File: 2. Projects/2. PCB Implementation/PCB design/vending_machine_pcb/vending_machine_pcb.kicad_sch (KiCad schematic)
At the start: 0 parts

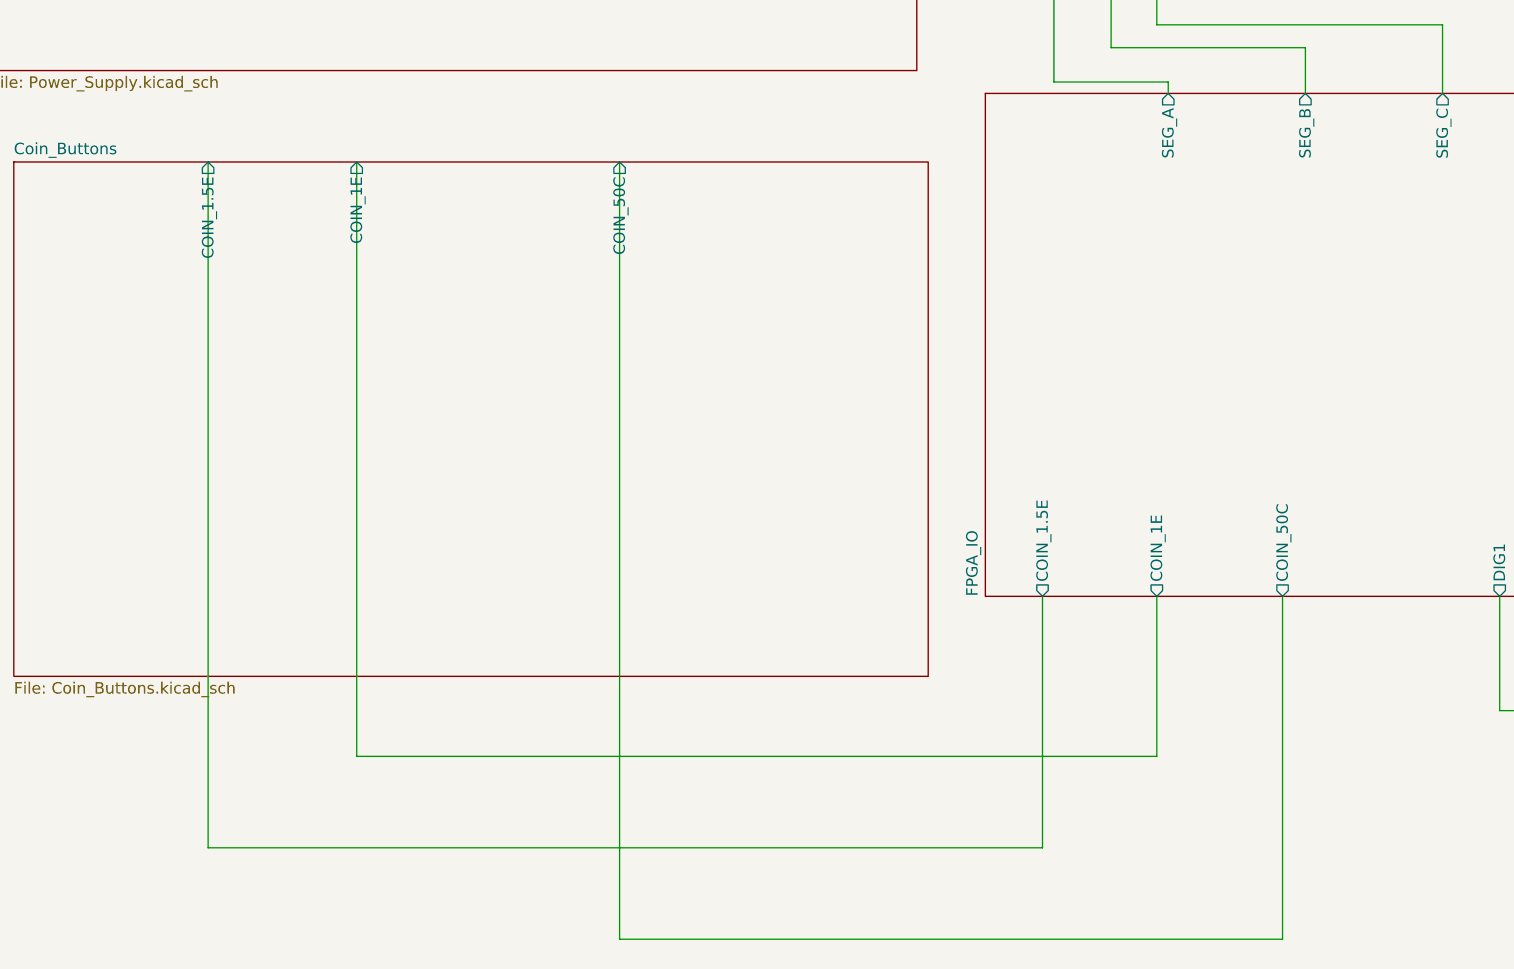
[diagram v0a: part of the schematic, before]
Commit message: PCB implementation
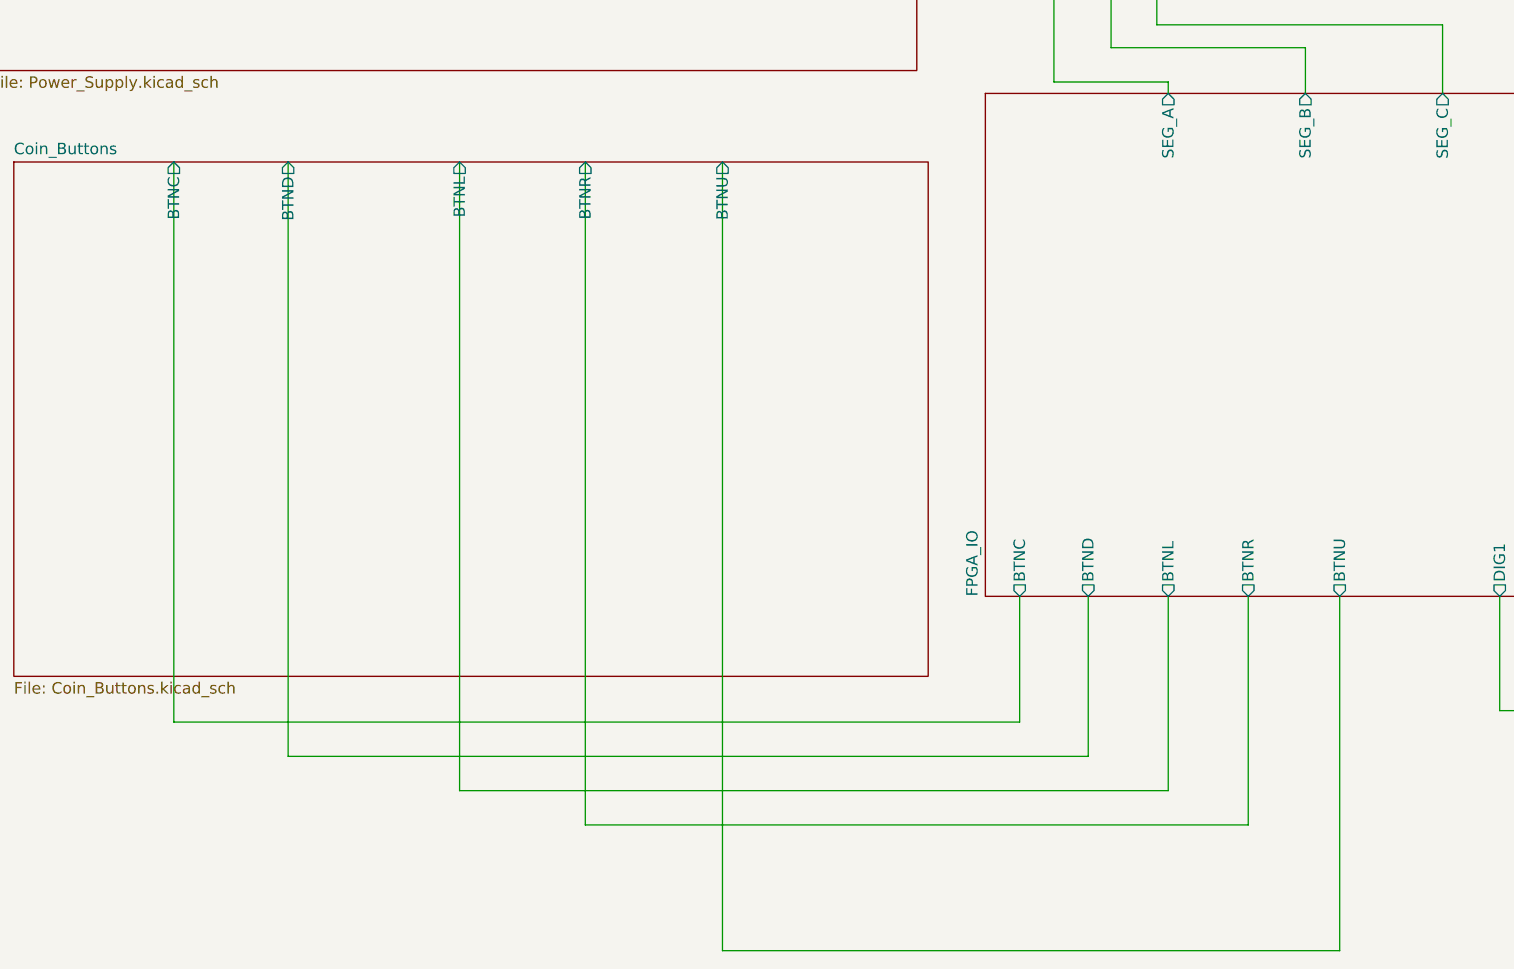
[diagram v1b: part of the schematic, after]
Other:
- sheet Coin_Buttons ports: added BTNC, BTND, BTNL, BTNR, BTNU; removed COIN_1.5E, COIN_1E, COIN_50C
- sheet FPGA_IO ports: added BTNC, BTND, BTNL, BTNR, BTNU; removed COIN_1.5E, COIN_1E, COIN_50C
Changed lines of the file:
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@@
 	(wire
 		(pts
-			(xy 156.21 189.23) (xy 156.21 151.13)
+			(xy 162.56 190.5) (xy 93.98 190.5)
 		)
 		(stroke
@@
 	(wire
 		(pts
+			(xy 78.74 176.53) (xy 152.4 176.53)
+		)
+		(stroke
+			(width 0)
+			(type default)
+		)
+	)
+	(wire
+		(pts
+			(xy 45.72 168.91) (xy 134.62 168.91)
+		)
+		(stroke
+			(width 0)
+			(type default)
+		)
+	)
+	(wire
+		(pts
 			(xy 137.16 90.17) (xy 158.75 90.17)
 		)
@@
 	(wire
 		(pts
-			(xy 53.34 102.87) (xy 53.34 168.91)
+			(xy 33.02 165.1) (xy 127 165.1)
+		)
+		(stroke
+			(width 0)
+			(type default)
+		)
+	)
+	(wire
+		(pts
+			(xy 127 165.1) (xy 127 151.13)
+		)
+		(stroke
+			(width 0)
+			(type default)
+		)
+	)
+	(wire
+		(pts
+			(xy 64.77 102.87) (xy 64.77 172.72)
+		)
+		(stroke
+			(width 0)
+			(type default)
+		)
+	)
+	(wire
+		(pts
+			(xy 162.56 151.13) (xy 162.56 190.5)
 		)
 		(stroke
@@
 	(wire
 		(pts
-			(xy 53.34 168.91) (xy 142.24 168.91)
-		)
-		(stroke
-			(width 0)
-			(type default)
-		)
-	)
-	(wire
-		(pts
 			(xy 130.81 21.59) (xy 130.81 93.98)
 		)
@@
 	(wire
 		(pts
+			(xy 64.77 172.72) (xy 143.51 172.72)
+		)
+		(stroke
+			(width 0)
+			(type default)
+		)
+	)
+	(wire
+		(pts
+			(xy 45.72 102.87) (xy 45.72 168.91)
+		)
+		(stroke
+			(width 0)
+			(type default)
+		)
+	)
+	(wire
+		(pts
 			(xy 226.06 157.48) (xy 226.06 151.13)
 		)
@@
 	(wire
 		(pts
+			(xy 93.98 190.5) (xy 93.98 102.87)
+		)
+		(stroke
+			(width 0)
+			(type default)
+		)
+	)
+	(wire
+		(pts
 			(xy 171.45 21.59) (xy 171.45 52.07)
 		)
@@
 	(wire
 		(pts
-			(xy 142.24 168.91) (xy 142.24 151.13)
-		)
-		(stroke
-			(width 0)
-			(type default)
-		)
-	)
-	(wire
-		(pts
 			(xy 143.51 93.98) (xy 143.51 95.25)
 		)
@@
 	(wire
 		(pts
-			(xy 129.54 179.07) (xy 36.83 179.07)
-		)
-		(stroke
-			(width 0)
-			(type default)
-		)
-	)
-	(wire
-		(pts
 			(xy 283.21 163.83) (xy 180.34 163.83)
 		)
@@
 	(wire
 		(pts
-			(xy 82.55 189.23) (xy 156.21 189.23)
-		)
-		(stroke
-			(width 0)
-			(type default)
-		)
-	)
-	(wire
-		(pts
-			(xy 36.83 179.07) (xy 36.83 102.87)
-		)
-		(stroke
-			(width 0)
-			(type default)
-		)
-	)
-	(wire
-		(pts
-			(xy 129.54 151.13) (xy 129.54 179.07)
+			(xy 33.02 102.87) (xy 33.02 165.1)
 		)
 		(stroke
@@
 	(wire
 		(pts
+			(xy 152.4 176.53) (xy 152.4 151.13)
+		)
+		(stroke
+			(width 0)
+			(type default)
+		)
+	)
+	(wire
+		(pts
 			(xy 276.86 157.48) (xy 226.06 157.48)
 		)
@@
 	(wire
 		(pts
+			(xy 78.74 102.87) (xy 78.74 176.53)
+		)
+		(stroke
+			(width 0)
+			(type default)
+		)
+	)
+	(wire
+		(pts
+			(xy 134.62 168.91) (xy 134.62 151.13)
+		)
+		(stroke
+			(width 0)
+			(type default)
+		)
+	)
+	(wire
+		(pts
 			(xy 200.66 161.29) (xy 280.67 161.29)
 		)
@@
 	(wire
 		(pts
+			(xy 143.51 172.72) (xy 143.51 151.13)
+		)
+		(stroke
+			(width 0)
+			(type default)
+		)
+	)
+	(wire
+		(pts
 			(xy 261.62 59.69) (xy 276.86 59.69)
 		)
@@
 		(pts
 			(xy 280.67 161.29) (xy 280.67 48.26)
-		)
-		(stroke
-			(width 0)
-			(type default)
-		)
-	)
-	(wire
-		(pts
-			(xy 82.55 102.87) (xy 82.55 189.23)
 		)
 		(stroke
@@
 			)
 		)
-		(pin "COIN_1.5E" output
-			(at 129.54 151.13 270)
-			(effects
-				(font
-					(size 1.27 1.27)
-				)
-				(justify left)
-			)
-		)
-		(pin "COIN_1E" output
-			(at 142.24 151.13 270)
-			(effects
-				(font
-					(size 1.27 1.27)
-				)
-				(justify left)
-			)
-		)
-		(pin "COIN_50C" output
-			(at 156.21 151.13 270)
+		(pin "BTNC" output
+			(at 127 151.13 270)
+			(effects
+				(font
+					(size 1.27 1.27)
+				)
+				(justify left)
+			)
+		)
+		(pin "BTND" output
+			(at 134.62 151.13 270)
+			(effects
+				(font
+					(size 1.27 1.27)
+				)
+				(justify left)
+			)
+		)
+		(pin "BTNL" output
+			(at 143.51 151.13 270)
+			(effects
+				(font
+					(size 1.27 1.27)
+				)
+				(justify left)
+			)
+		)
+		(pin "BTNR" output
+			(at 152.4 151.13 270)
+			(effects
+				(font
+					(size 1.27 1.27)
+				)
+				(justify left)
+			)
+		)
+		(pin "BTNU" output
+			(at 162.56 151.13 270)
 			(effects
 				(font
@@
 			)
 		)
-		(pin "COIN_1.5E" output
-			(at 36.83 102.87 90)
-			(effects
-				(font
-					(size 1.27 1.27)
-				)
-				(justify right)
-			)
-		)
-		(pin "COIN_1E" output
-			(at 53.34 102.87 90)
-			(effects
-				(font
-					(size 1.27 1.27)
-				)
-				(justify right)
-			)
-		)
-		(pin "COIN_50C" output
-			(at 82.55 102.87 90)
-			(effects
-				(font
+		(pin "BTNC" output
+			(at 33.02 102.87 90)
+			(effects
+				(font
+					(size 1.27 1.27)
+				)
+				(justify right)
+			)
+		)
+		(pin "BTND" output
+			(at 45.72 102.87 90)
+			(effects
+				(font
+					(size 1.27 1.27)
+				)
+				(justify right)
+			)
+		)
+		(pin "BTNL" output
+			(at 64.77 102.87 90)
+			(effects
+				(font
+					(size 1.27 1.27)
+				)
+				(justify right)
+			)
+		)
+		(pin "BTNR" output
+			(at 78.74 102.87 90)
+			(effects
+				(font
+					(size 1.27 1.27)
+				)
+				(justify right)
+			)
+		)
+		(pin "BTNU" output
+			(at 93.98 102.87 90)
+			(effects
+				(font
